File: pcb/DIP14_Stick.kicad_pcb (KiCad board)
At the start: 2 copper layers, 146 x 34.5 mm, 42 parts, among them J1 PinHeader_1x10_P2.54mm_Horizo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, J2 PinHeader_1x10_P2.54mm_Horizo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

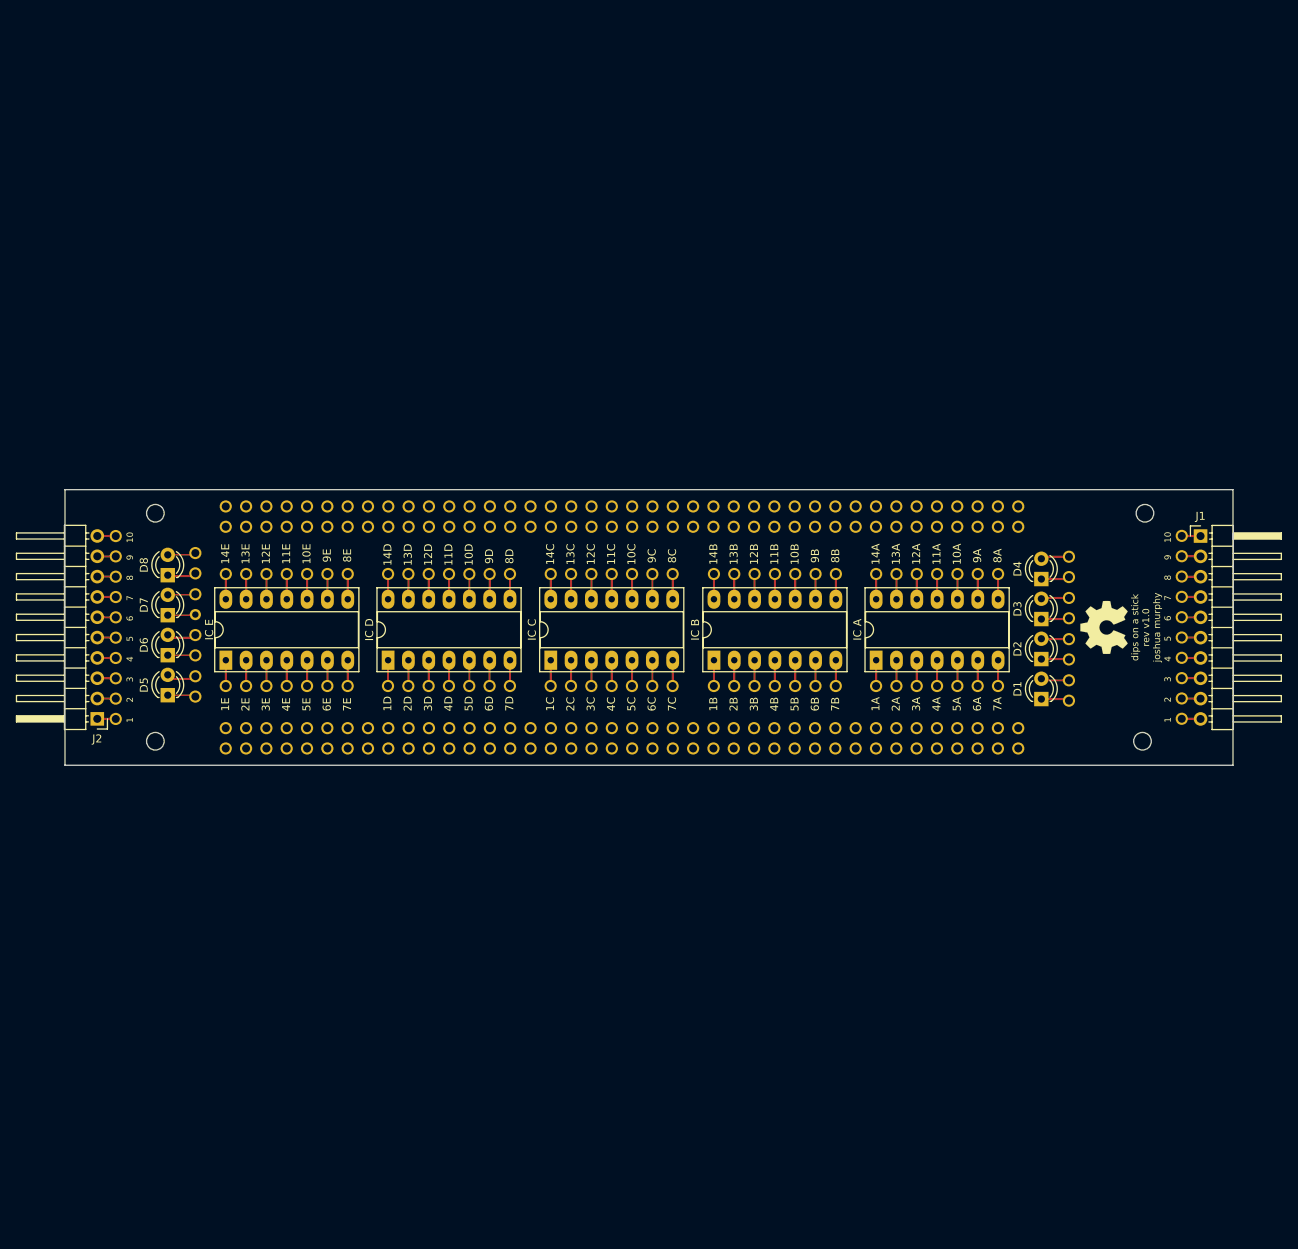
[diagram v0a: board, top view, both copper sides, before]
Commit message: A revision prototype that I already don't like
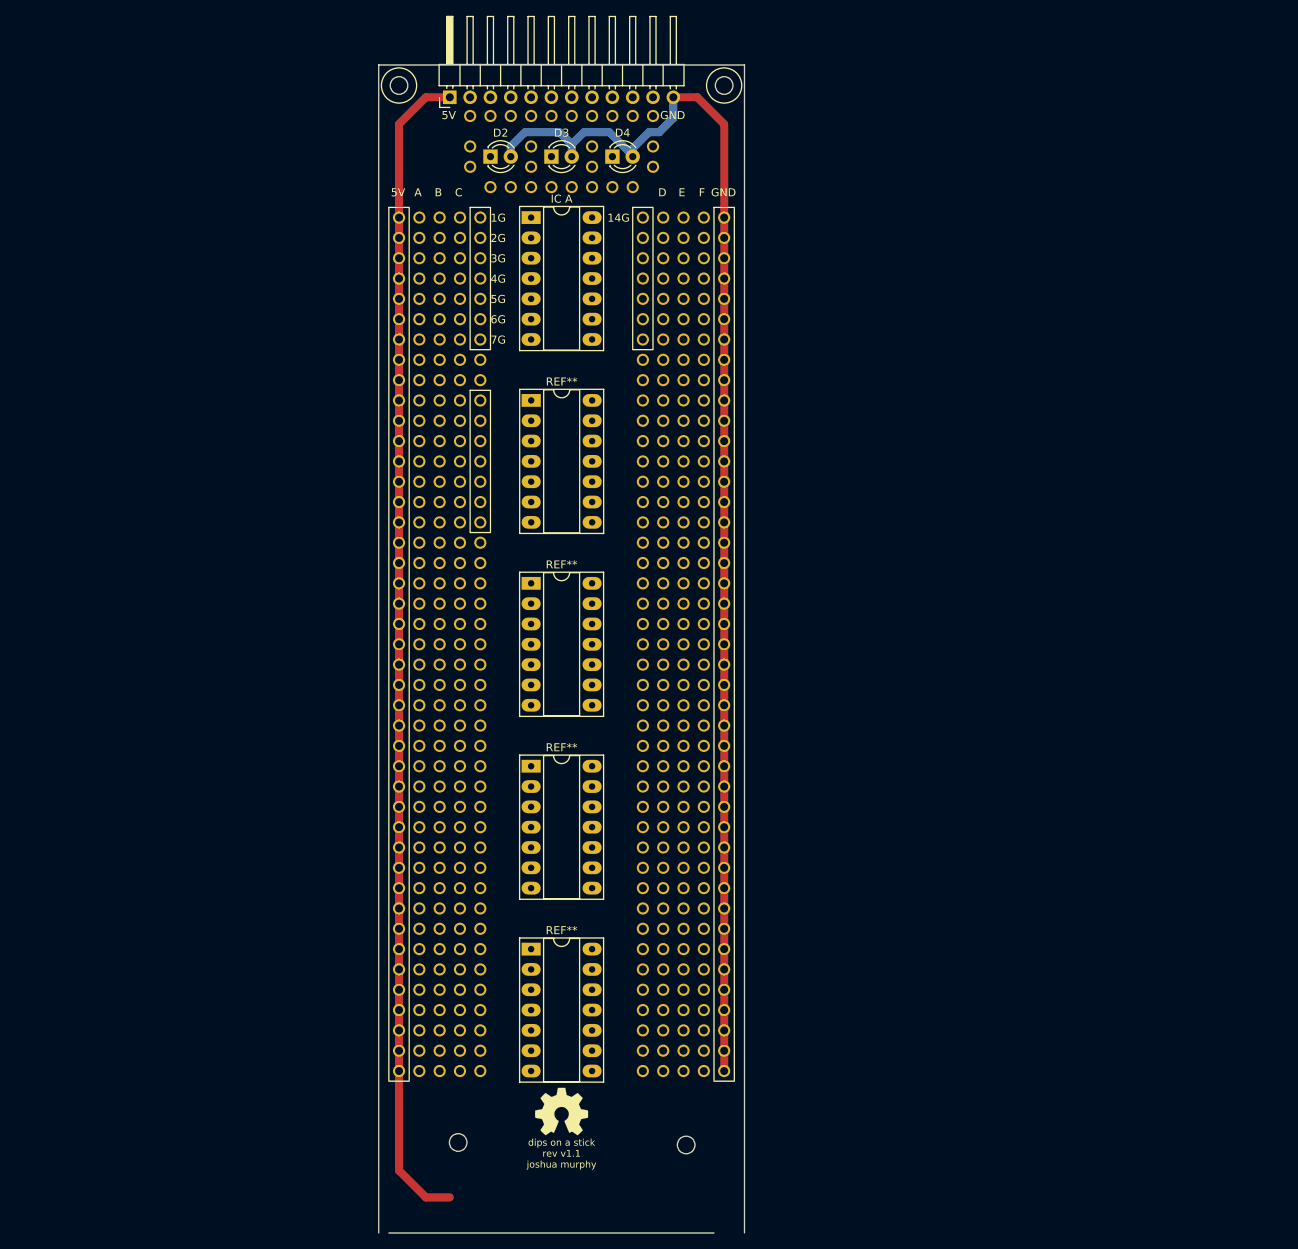
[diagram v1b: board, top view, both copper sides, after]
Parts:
- removed ?: 1x7_Right_Side_IC_Pinout, DIP14_Stick:1x7_Right_Side_IC_Pinout
- removed D1, D5, D6, D7, D8: LED_D3.0mm, DIP14_Stick:LED_D3.0mm
- removed IC B: DIP-14_W7.62mm_Socket_LongPads, Package_DIP:DIP-14_W7.62mm_Socket_LongPads
- removed IC C: DIP-14_W7.62mm_Socket_LongPads, Package_DIP:DIP-14_W7.62mm_Socket_LongPads
- removed IC D: DIP-14_W7.62mm_Socket_LongPads, Package_DIP:DIP-14_W7.62mm_Socket_LongPads
- removed IC E: DIP-14_W7.62mm_Socket_LongPads, Package_DIP:DIP-14_W7.62mm_Socket_LongPads
- removed J1: PinHeader_1x10_P2.54mm_Horizontal, Connector_PinHeader_2.54mm:PinHeader_1x10_P2.54mm_Horizontal
- removed the REF** at (90.1, 111.9)
- removed the REF** at (86.3, 108.1)
- removed the REF** at (90.1, 119.7)
- removed the REF** at (90.1, 97.9)
- removed the REF** at (171.4, 111.9)
- removed the REF** at (90.1, 92.0)
- removed the REF** at (86.3, 103.0)
- removed the REF** at (86.3, 97.8)
- removed the REF** at (86.3, 113.2)
- removed the REF** at (195.5, 108.6)
- removed the REF** at (81.3, 118.8)
- removed the REF** at (76.3, 105.2)
- removed the REF** at (151.1, 97.9)
- removed the REF** at (110.4, 97.9)
- removed the REF** at (195.5, 98.3)
- removed the REF** at (209.6, 103.9)
- removed the REF** at (81.3, 90.3)
- removed the REF** at (151.1, 111.9)
- removed the REF** at (130.7, 97.9)
- removed the REF** at (195.5, 103.4)
- removed the REF** at (195.5, 113.7)
- removed the REF** at (110.4, 111.9)
- removed the REF** at (130.7, 111.9)
- added REF**: DIP-14_W7.62mm_Socket_LongPads, Package_DIP:DIP-14_W7.62mm_Socket_LongPads, F.Cu at (128.3, 121.9)
- added REF**: DIP14 Stick Protoboard, DIP14_Stick:DIP14 Stick Protoboard, F.Cu at (111.8, 40.6)
- added REF**: DIP-14_W7.62mm_Socket_LongPads, Package_DIP:DIP-14_W7.62mm_Socket_LongPads, F.Cu at (128.3, 76.2)
- added REF**: MountingHole_2.2mm_M2, MountingHole:MountingHole_2.2mm_M2, F.Cu at (111.8, 36.8)
- added REF**: DIP-14_W7.62mm_Socket_LongPads, Package_DIP:DIP-14_W7.62mm_Socket_LongPads, F.Cu at (128.3, 144.8)
- added REF**: DIP-14_W7.62mm_Socket_LongPads, Package_DIP:DIP-14_W7.62mm_Socket_LongPads, F.Cu at (128.3, 99.1)
- added REF**: OSHW-Symbol_6.7x6mm_SilkScreen, Symbol:OSHW-Symbol_6.7x6mm_SilkScreen, F.Cu at (132.1, 165.1)
- added REF**: MountingHole_2.2mm_M2, MountingHole:MountingHole_2.2mm_M2, F.Cu at (152.4, 36.8)
- D2, D3, D4: footprint DIP14_Stick:LED_D3.0mm -> LED_THT:LED_D3.0mm
- J2: value PinHeader_1x10_P2.54mm_Horizontal -> PinHeader_1x12_P2.54mm_Horizontal; footprint Connector_PinHeader_2.54mm:PinHeader_1x10_P2.54mm_Horizontal -> Connector_PinHeader_2.54mm:PinHeader_1x12_P2.54mm_Horizontal
- REF**: moved to B.Cu
- moved REF** 99.2 mm to (119.2, 169.0), turned to 90 degrees
- moved REF** 97.6 mm to (147.7, 169.3), turned to 90 degrees
- moved D2 93.2 mm to (123.2, 45.7), turned to 0 degrees
- moved REF** 90.9 mm to (132.1, 165.1), turned to 180 degrees
- moved J2 89.3 mm to (118.1, 38.3), turned to 90 degrees
- moved D3 84.2 mm to (130.8, 45.7), turned to 0 degrees
- moved D4 75.3 mm to (138.4, 45.7), turned to 0 degrees
- moved IC A 70.2 mm to (128.3, 53.3), turned to 0 degrees
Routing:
- net (no net): track 327.0 -> 304.0 mm
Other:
- board size 146 x 34.5 mm -> 45.7 x 146 mm
- board text added: "5V"
- board text added: "GND"
- board text added: "dips on a stick rev v1.1 joshua murphy"
- board text removed: "dips on a stick rev v1.0 joshua murphy"
